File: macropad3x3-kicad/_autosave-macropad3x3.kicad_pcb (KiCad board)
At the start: 2 copper layers, 77 x 112.5 mm, 26 parts, among them J1 OLED-4PIN, U1 Arduino_Pro_Micro

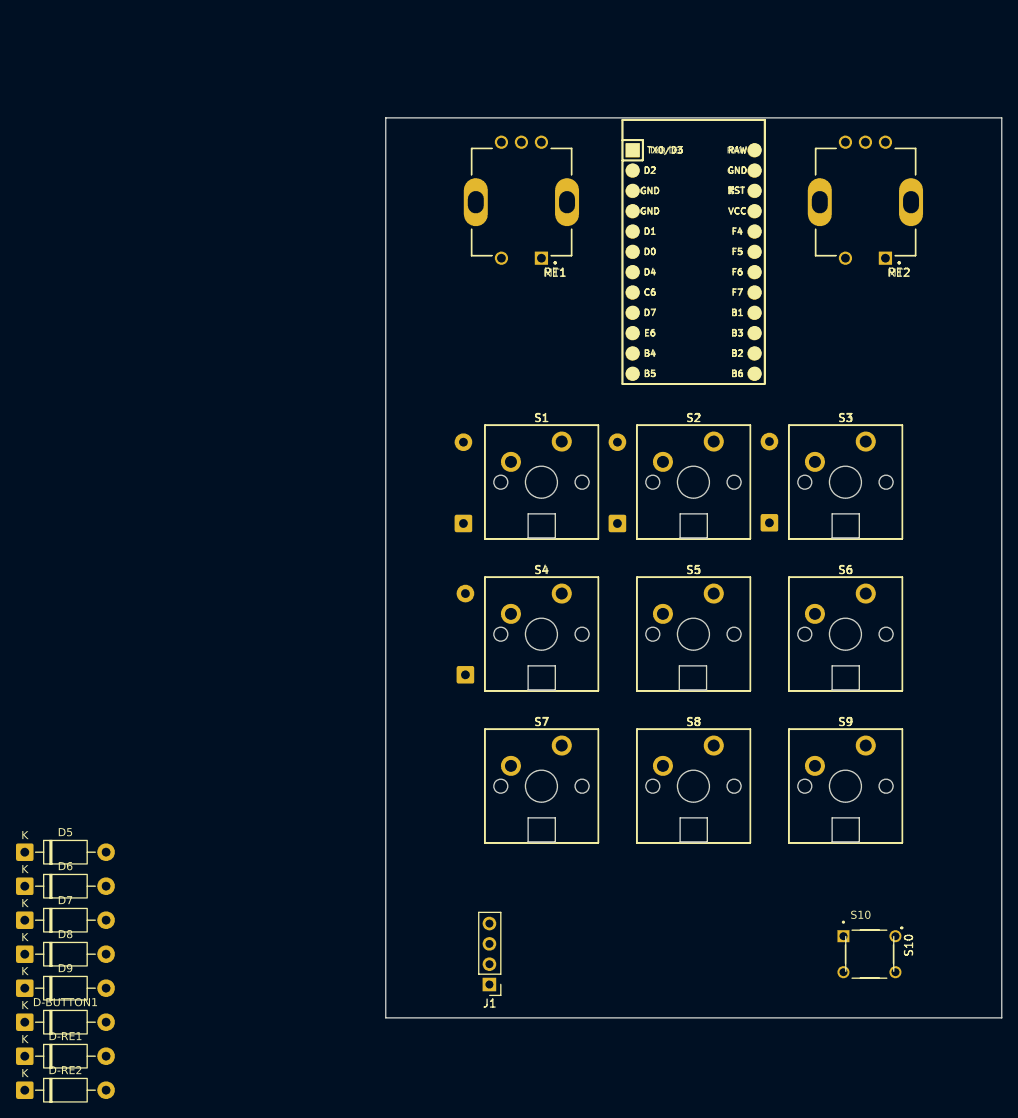
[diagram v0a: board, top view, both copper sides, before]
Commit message: added stuff
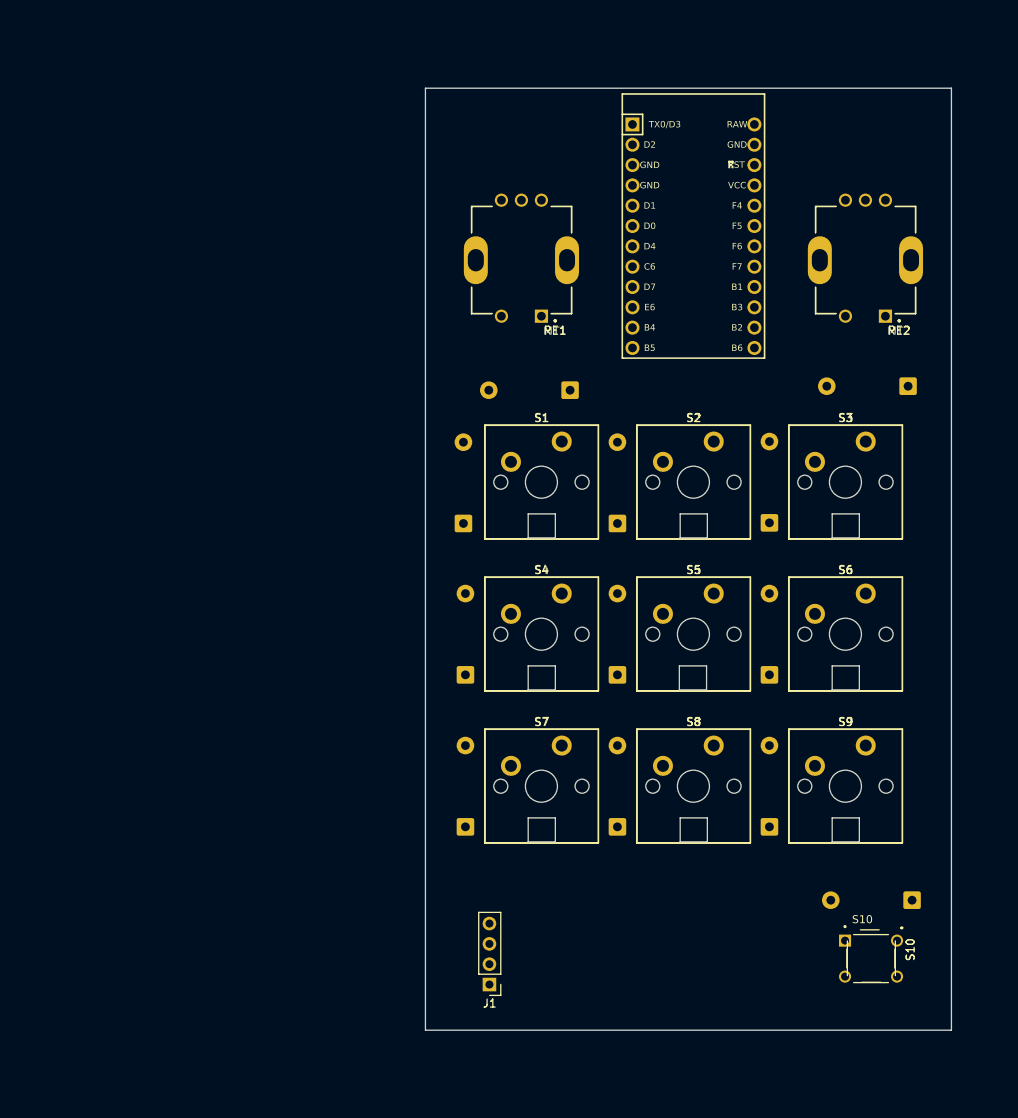
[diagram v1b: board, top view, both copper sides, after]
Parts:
- D-BUTTON1, D-RE1, D-RE2, D5, D6, D7, D8, D9: moved to B.Cu
- moved D-RE2 141.2 mm to (157.8, 84.2), turned to 180 degrees
- moved D-BUTTON1 112.0 mm to (158.3, 148.5), turned to 180 degrees
- moved D-RE1 107.6 mm to (115.6, 84.8), turned to 180 degrees
- moved D6 96.8 mm to (140.5, 120.3), turned to 90 degrees
- moved D9 95.2 mm to (140.5, 139.3), turned to 90 degrees
- moved D5 77.3 mm to (121.5, 120.3), turned to 90 degrees
- moved D8 75.8 mm to (121.5, 139.3), turned to 90 degrees
- moved D7 56.3 mm to (102.5, 139.3), turned to 90 degrees
- moved MT1 7.25 mm to (109.5, 68.5)
- moved MT2 7.25 mm to (152.5, 68.5)
- moved U1 3.25 mm to (131.0, 65.5)
- moved S10 0.59 mm to (153.2, 155.8)
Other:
- board size 77 x 112.5 mm -> 65.8 x 117.8 mm

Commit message: hi
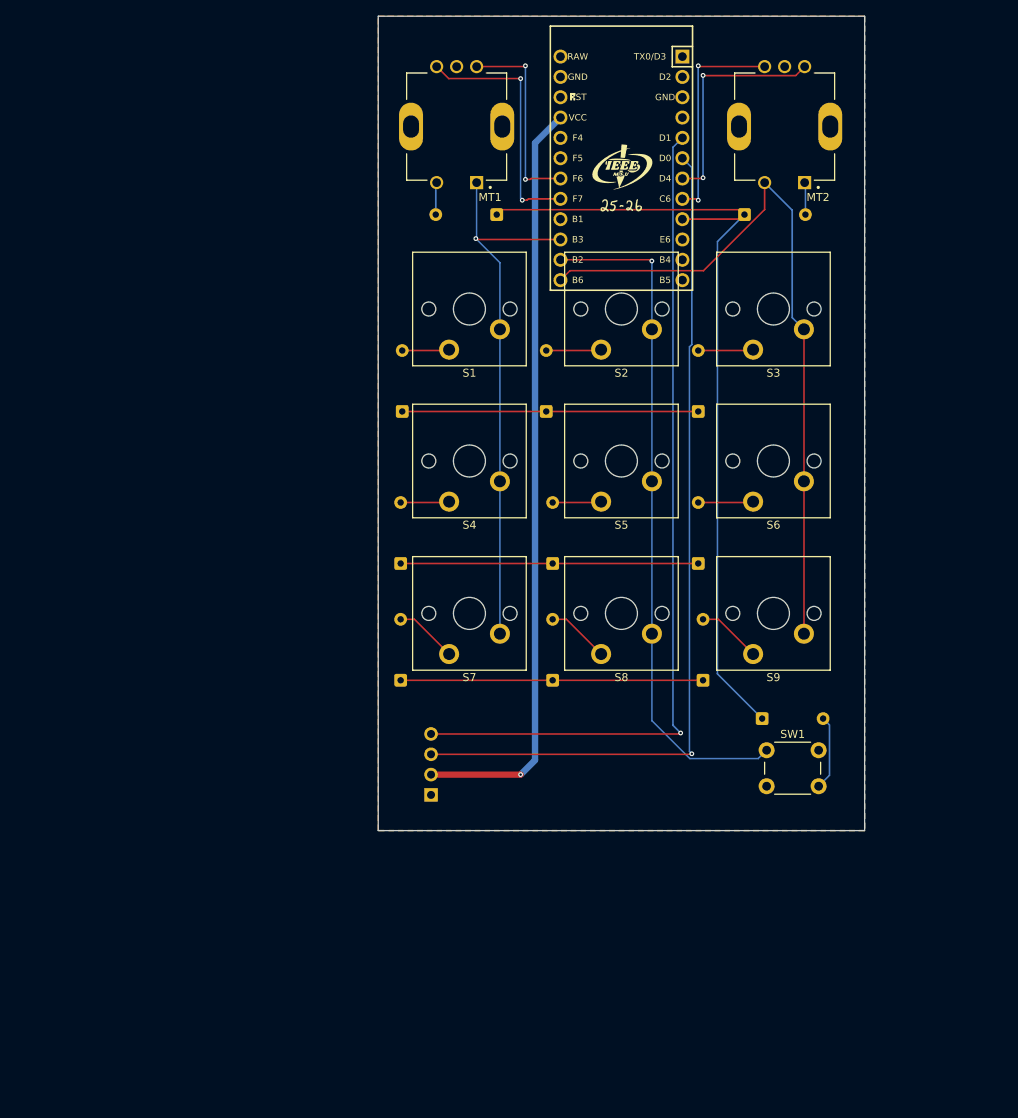
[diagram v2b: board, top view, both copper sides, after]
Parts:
- removed S10: TS02-66-95-BK-260-LCR-D, macropad:SW_TS02-66-95-BK-260-LCR-D
- added SW1: SW_Push_45deg, Button_Switch_THT:SW_PUSH_6mm, F.Cu at (140.2, 129.8)
- D-BUTTON1, D-RE1, D-RE2, D1, D2, D3, D4, D5, D6, D7, D8, D9: value Diode -> 1N4148; footprint Diode_THT:D_DO-41_SOD81_P10.16mm_Horizontal -> Diode_THT:D_DO-35_SOD27_P7.62mm_Horizontal
- J1: value OLED-4PIN -> OLED_128x32
- U1: moved to B.Cu
- moved D-RE2 29.6 mm to (137.4, 62.8), turned to 0 degrees
- moved D-BUTTON1 29.4 mm to (139.6, 125.8), turned to 0 degrees
- moved J1 24.8 mm to (96.6, 125.5)
- moved D-RE1 23.8 mm to (106.4, 62.8)
- moved S1 23.4 mm to (103.0, 74.6), turned to 180 degrees
- moved S2 23.4 mm to (122.0, 74.6), turned to 180 degrees
- moved S3 23.4 mm to (141.0, 74.6), turned to 180 degrees
- moved S4 23.4 mm to (103.0, 93.6), turned to 180 degrees
- moved S5 23.4 mm to (122.0, 93.6), turned to 180 degrees
- moved S6 23.4 mm to (141.0, 93.6), turned to 180 degrees
- moved S7 23.4 mm to (103.0, 112.7), turned to 180 degrees
- moved S8 23.4 mm to (122.0, 112.7), turned to 180 degrees
- moved S9 23.4 mm to (141.0, 112.7), turned to 180 degrees
- moved D9 20.1 mm to (132.2, 121.0)
- moved D7 20.0 mm to (94.4, 121.0)
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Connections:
- D-RE2 pad 2: /RE2-2 -> /RE2-1
- J1 pad 1: (no net) -> GND
- J1 pad 2: (no net) -> +5V
- J1 pad 3: (no net) -> /SCL
- J1 pad 4: (no net) -> /SDA
- MT1 pad 1: /RE1-1 -> /col0
- MT1 pad A: unconnected-(MT1-PadA) -> /RE1A
- MT1 pad B: unconnected-(MT1-PadB) -> /RE1B
- MT2 pad 2: /RE2-2 -> /col2
- MT2 pad A: unconnected-(MT2-PadA) -> /RE2A
- MT2 pad B: unconnected-(MT2-PadB) -> /RE2B
- S1 pad 1: /RE1-1 -> /col0
- S2 pad 1: /Button1 -> /col1
- S3 pad 1: /RE2-1 -> /col2
- S4 pad 1: /RE1-1 -> /col0
- S5 pad 1: /Button1 -> /col1
- S6 pad 1: /RE2-1 -> /col2
- S7 pad 1: /RE1-1 -> /col0
- S8 pad 1: /Button1 -> /col1
- S9 pad 1: /RE2-1 -> /col2
- U1 pad 10: unconnected-(U1-7/PE6-Pad10) -> /row1
- U1 pad 11: unconnected-(U1-8/PB4-Pad11) -> /row2
- U1 pad 12: unconnected-(U1-9/PB5-Pad12) -> /row3
- U1 pad 13: unconnected-(U1-10/PB6-Pad13) -> /col2
- U1 pad 14: unconnected-(U1-16/PB2-Pad14) -> /col1
- U1 pad 15: unconnected-(U1-14/PB3-Pad15) -> /col0
- U1 pad 17: unconnected-(U1-A0/PF7-Pad17) -> /RE1B
- U1 pad 18: unconnected-(U1-A1/PF6-Pad18) -> /RE1A
- U1 pad 23: unconnected-(U1-GND-Pad23) -> GND
- U1 pad 3: unconnected-(U1-GND-Pad3) -> GND
- U1 pad 4: unconnected-(U1-GND-Pad4) -> GND
- U1 pad 5: (no net) -> /SDA
- U1 pad 6: (no net) -> /SCL
- U1 pad 7: unconnected-(U1-4/PD4-Pad7) -> /RE2A
- U1 pad 8: unconnected-(U1-5/PC6-Pad8) -> /RE2B
- U1 pad 9: unconnected-(U1-6/PD7-Pad9) -> /row0
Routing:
- net /SCL: track 0.00 -> 107.8 mm, vias 0 -> 1
- net /SDA: track 0.00 -> 106.5 mm, vias 0 -> 1
- net /row0: track 0.00 -> 106.2 mm
- net +5V: track 0.00 -> 95.4 mm, vias 0 -> 1
- net /col2: track 0.00 -> 91.0 mm
- net /col1: track 0.00 -> 85.7 mm, vias 0 -> 1
- net /col0: track 0.00 -> 68.3 mm, vias 0 -> 1
- net /row3: track 0.00 -> 37.8 mm
- net /row2: track 0.00 -> 37.2 mm
- net /row1: track 0.00 -> 37.0 mm
- net /RE1B: track 0.00 -> 31.3 mm, vias 0 -> 2
- net /RE2A: track 0.00 -> 28.6 mm, vias 0 -> 2
- net /RE2B: track 0.00 -> 27.2 mm, vias 0 -> 2
- net /RE1A: track 0.00 -> 24.8 mm, vias 0 -> 2
- net /Button2: track 0.00 -> 9.34 mm
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- added copper zone on B.Cu, net GND
- added copper zone on F.Cu, net GND
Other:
- board size 65.8 x 117.8 mm -> 60.8 x 101.8 mm
